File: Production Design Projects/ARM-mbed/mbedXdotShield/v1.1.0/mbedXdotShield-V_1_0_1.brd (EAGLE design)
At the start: 81.3 x 53.3 mm, 70 parts, among them CON1 47346-0001, CON2 S2B-PH-SM4-TB(LF)(SN), Q1 12MHz, SW3 JS202011JCQN, T1 BSS84, U1 MTXDOT-EU1-A00-1, U2 TLV73333PDBVT, U3 AT45DB321E-SHF-B

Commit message: Added v1.1.0 updated schematic. R3:1.5K->220R, R13,R14:470R->1.5K, rerouted UART1_, moved USB micro into board, placed resistors R14-to-R27 on front of PCB (no components on rear)
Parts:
- R11: value 1.5K -> 470R
- R12, R13: value 2K -> 1.5K
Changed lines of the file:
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@@
 <element name="R8" library="mbed-HDK-RLCQ" package="0402" value="1.5K" x="8.6868" y="-103.3272" rot="R90"/>
 <element name="R10" library="mbed-HDK-RLCQ" package="0402" value="10K" x="11.43" y="-112.1664" rot="R90"/>
-<element name="R11" library="mbed-HDK-RLCQ" package="0402" value="1.5K" x="1.8288" y="-108.204"/>
-<element name="R12" library="mbed-HDK-RLCQ" package="0402" value="2K" x="1.8288" y="-110.3376"/>
-<element name="R13" library="mbed-HDK-RLCQ" package="0402" value="2K" x="1.8288" y="-112.4712"/>
+<element name="R11" library="mbed-HDK-RLCQ" package="0402" value="470R" x="1.8288" y="-108.204"/>
+<element name="R12" library="mbed-HDK-RLCQ" package="0402" value="1.5K" x="1.8288" y="-110.3376"/>
+<element name="R13" library="mbed-HDK-RLCQ" package="0402" value="1.5K" x="1.8288" y="-112.4712"/>
 <element name="R9" library="mbed-HDK-RLCQ" package="0402" value="10K" x="3.2004" y="-115.6716" rot="R180"/>
 <element name="LED3" library="mbed-HDK-Optical" package="CHIPLED_0603" value="RED" x="1.8288" y="-107.1372" smashed="yes" rot="R90">

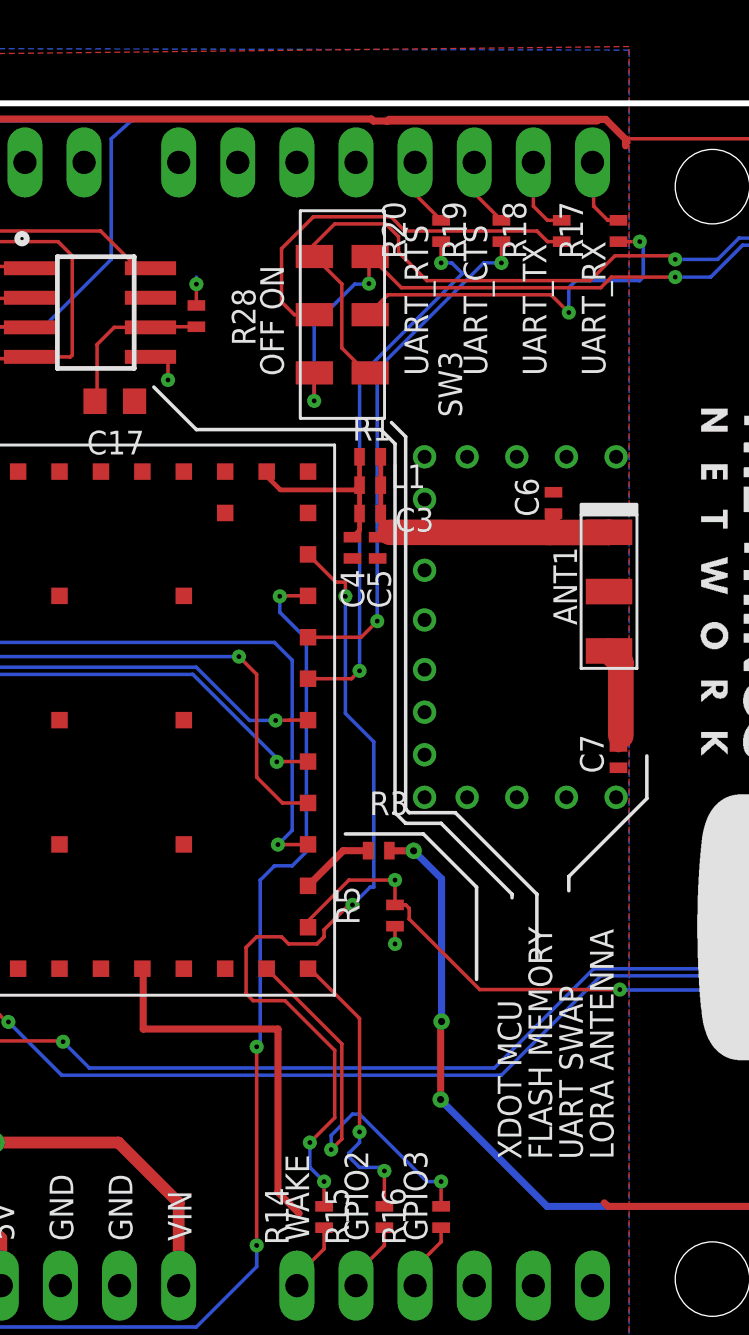
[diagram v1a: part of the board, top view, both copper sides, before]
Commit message: Added v1.1.0, see readme
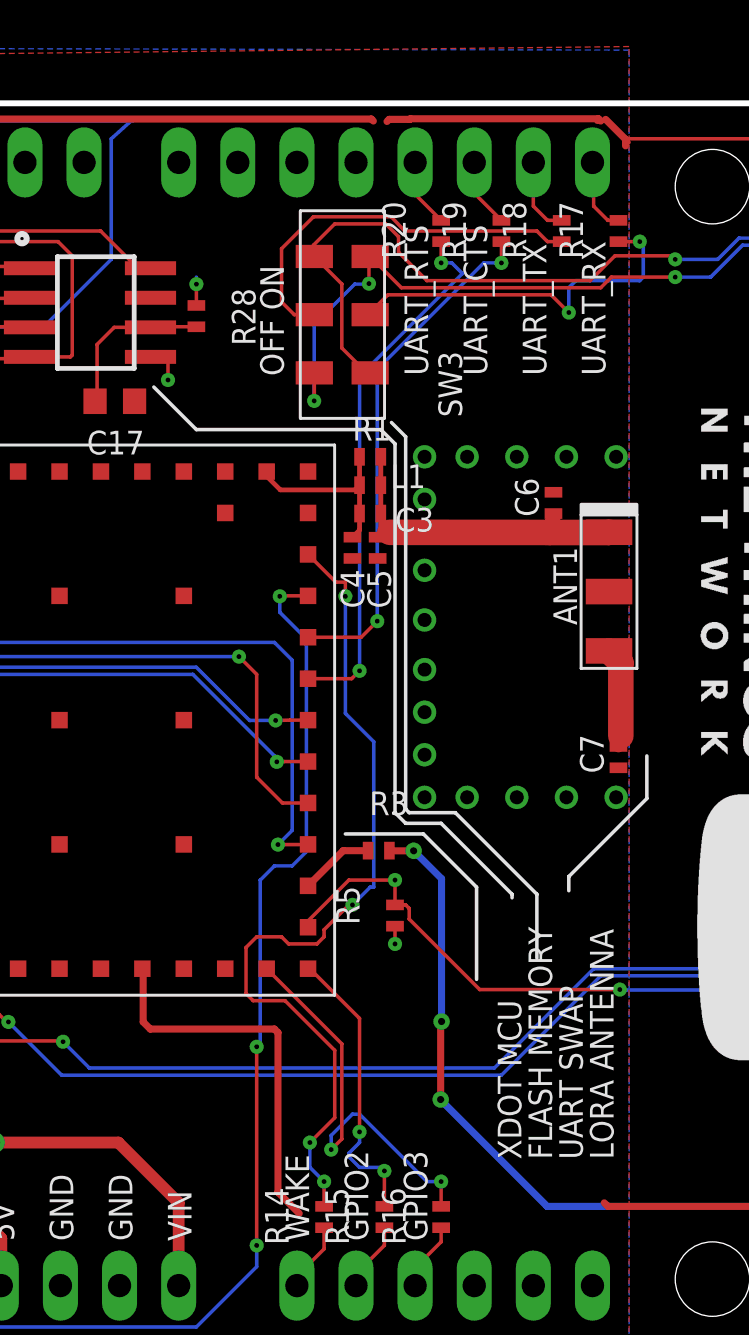
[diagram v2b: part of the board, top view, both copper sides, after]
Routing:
- net GND: track 129.4 -> 119.3 mm
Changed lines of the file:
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@@
 <wire x1="63.246" y1="-135.1788" x2="63.0936" y2="-135.0264" width="0.3048" layer="1"/>
 <wire x1="49.9872" y1="-135.4836" x2="49.0728" y2="-134.5692" width="0.3048" layer="1"/>
-<wire x1="49.0728" y1="-134.5692" x2="49.0728" y2="-127.5588" width="0.3048" layer="1"/>
-<wire x1="49.0728" y1="-127.5588" x2="43.2816" y2="-127.5588" width="0.3048" layer="1"/>
-<wire x1="43.2816" y1="-127.5588" x2="43.2816" y2="-125.0004" width="0.3048" layer="1"/>
+<wire x1="43.2816" y1="-127.254" x2="43.2816" y2="-125.0004" width="0.3048" layer="1"/>
 <wire x1="43.2816" y1="-125.0004" x2="43.2468" y2="-124.9656" width="0.3048" layer="1"/>
 <wire x1="76.6236" y1="-91.44" x2="76.6236" y2="-90.492" width="0.1524" layer="1"/>
@@
 <wire x1="64.008" y1="-89.6112" x2="64.008" y2="-89.32855" width="0.3048" layer="1"/>
 <wire x1="64.008" y1="-89.32855" x2="63.152578125" y2="-88.473128125" width="0.3048" layer="1"/>
-<wire x1="63.152578125" y1="-88.473128125" x2="53.848" y2="-88.473128125" width="0.3048" layer="1"/>
 <wire x1="53.848" y1="-88.473128125" x2="53.75701875" y2="-88.564109375" width="0.3048" layer="1"/>
-<wire x1="62.7888" y1="-88.5444" x2="53.171853125" y2="-88.5444" width="0.3048" layer="1"/>
 <wire x1="53.171853125" y1="-88.5444" x2="53.086103125" y2="-88.45865" width="0.3048" layer="1"/>
 <wire x1="53.086103125" y1="-88.45865" x2="36.81415" y2="-88.45865" width="0.3048" layer="1"/>
 <wire x1="36.81415" y1="-88.45865" x2="36.7284" y2="-88.5444" width="0.3048" layer="1"/>
+<wire x1="49.0728" y1="-134.5692" x2="49.0728" y2="-127.7112" width="0.3048" layer="1"/>
+<wire x1="49.0728" y1="-127.7112" x2="48.9204" y2="-127.5588" width="0.3048" layer="1"/>
+<wire x1="48.9204" y1="-127.5588" x2="43.5864" y2="-127.5588" width="0.3048" layer="1"/>
+<wire x1="43.5864" y1="-127.5588" x2="43.2816" y2="-127.254" width="0.3048" layer="1"/>
+<wire x1="53.848" y1="-88.473128125" x2="54.735271875" y2="-88.473128125" width="0.3048" layer="1"/>
+<wire x1="54.735271875" y1="-88.473128125" x2="54.76123125" y2="-88.44716875" width="0.3048" layer="1"/>
+<wire x1="54.76123125" y1="-88.44716875" x2="62.84396875" y2="-88.44716875" width="0.3048" layer="1"/>
+<wire x1="62.84396875" y1="-88.44716875" x2="62.9412" y2="-88.5444" width="0.3048" layer="1"/>
+<wire x1="62.84396875" y1="-88.44716875" x2="62.81231875" y2="-88.5444" width="0" layer="19" extent="1-1"/>
 </signal>
 <signal name="RFU1">
